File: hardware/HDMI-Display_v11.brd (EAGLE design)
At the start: 52 x 52 mm, 107 parts, among them IC1 TFP401A-PAD, IC2 24LC02B, IC3 IS31BL3506A-TTLS2, IC4 ATMEGA32U4-MU, IC5 LDO-TS1117CW-3V3, J20_1 JUMPER2-0402, J20_2 JUMPER2-0402, J30_1 JUMPER2-0402, J30_2 JUMPER2-0402, Q1 16MHz, SW1 SW-TACTILE-PTS840P, T6 BSS138PS, T7 BSS138PS, T8 BSS138PS, X1 PASSER-07, X2 PASSER-07, X3 PASSER-07, X4 PASSER-07

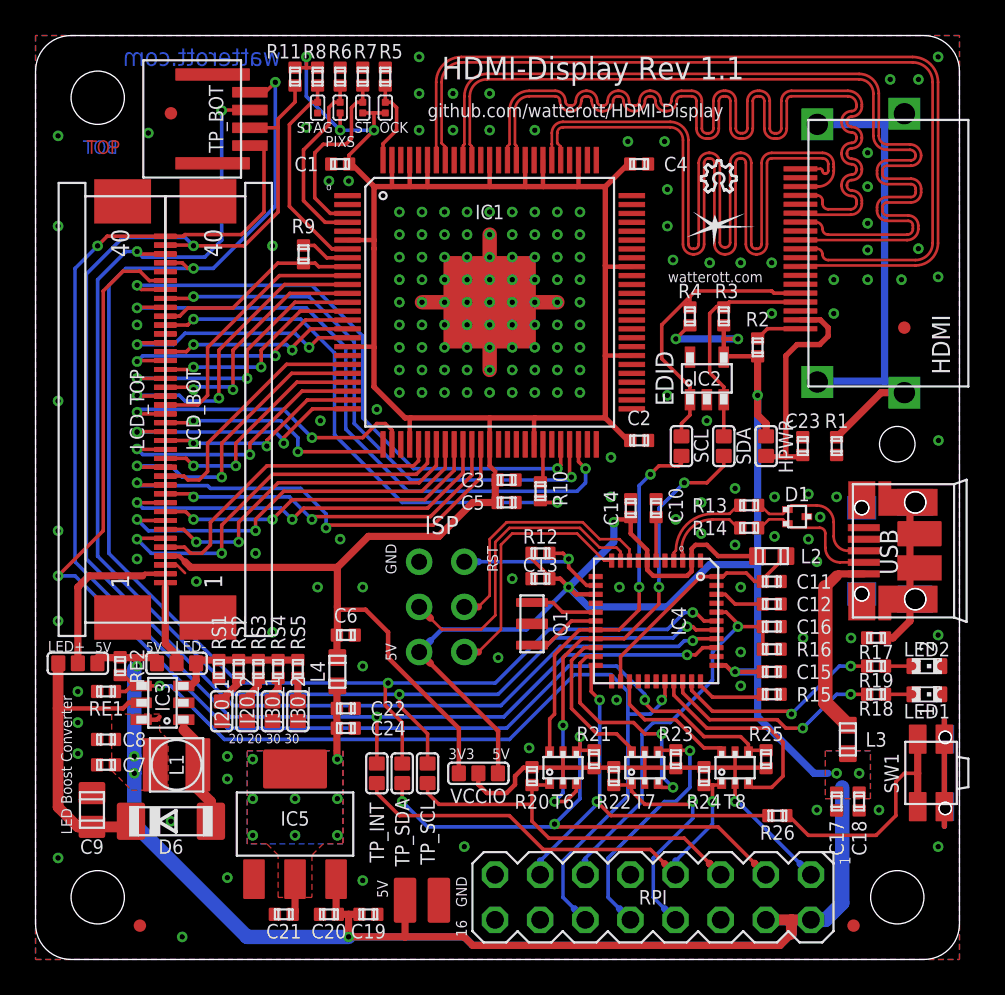
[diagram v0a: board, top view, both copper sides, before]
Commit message: updated schematics and layout
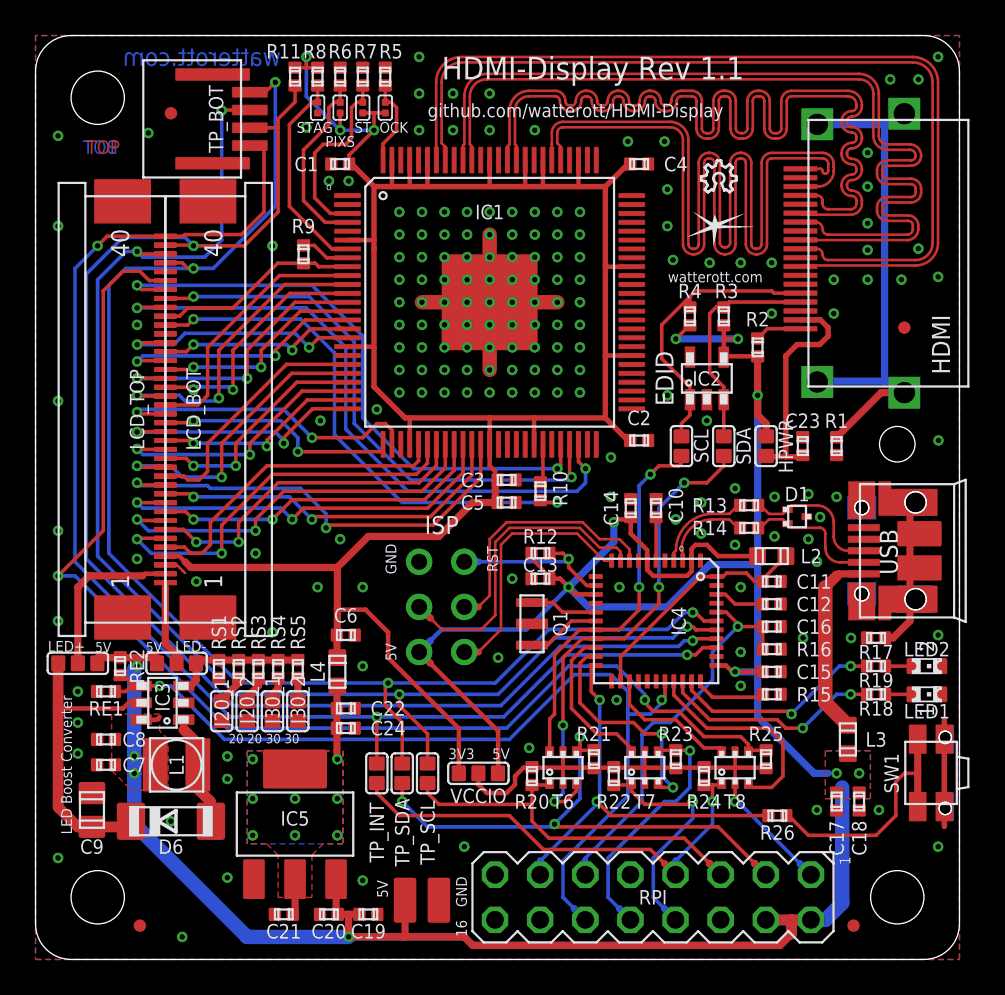
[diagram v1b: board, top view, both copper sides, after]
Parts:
- ISP: device we-board:ISP -> we-board:ISP-2X3
- L3, L4: value Ferrit@1A -> BLM18PG221SH1D
- USB: value USB-MICRO -> USB-MICROB; device we-con:USB-MICRO-10103594 -> we-con:USB-MICROB-10103594
